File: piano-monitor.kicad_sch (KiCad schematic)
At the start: 9 parts, among them J2 C14, J3 R, J4 DC, J5 230AC, J6 L

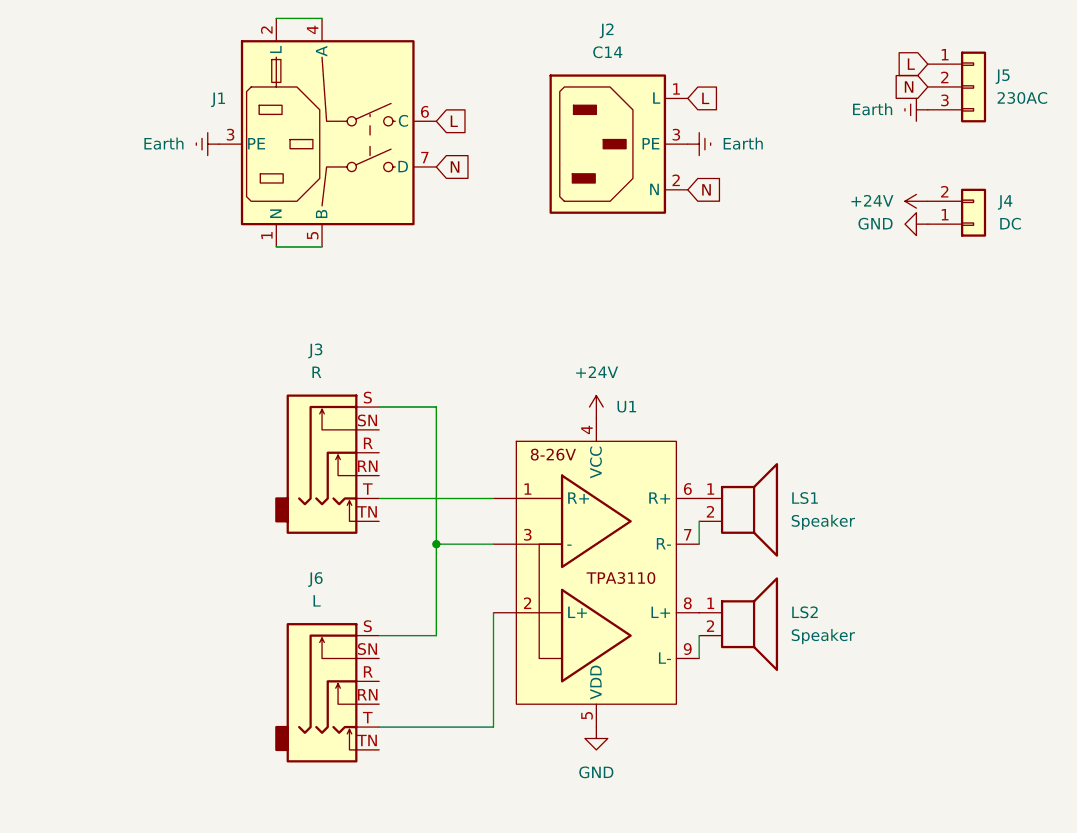
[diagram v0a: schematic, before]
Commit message: Update Schematic
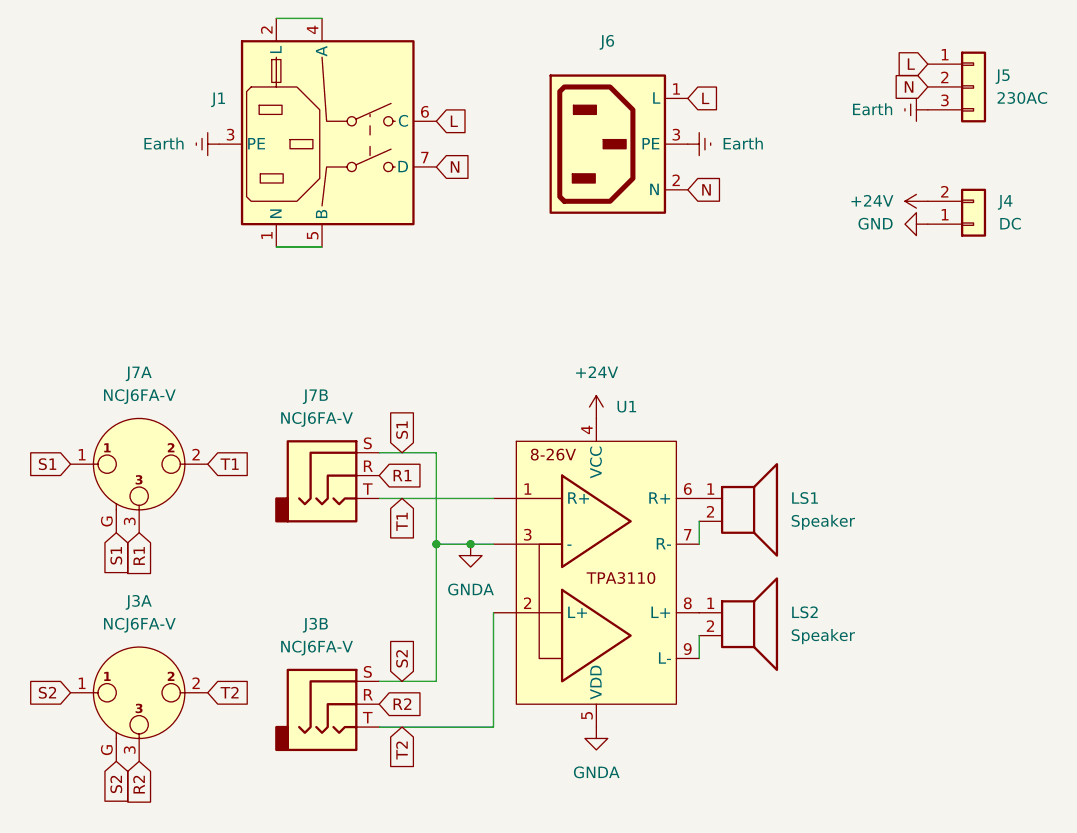
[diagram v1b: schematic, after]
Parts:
- removed J2: C14, symbol Connector:IEC_60320_C14_Receptacle
- removed J3: R, symbol Connector_Audio:AudioJack3_Switch
- removed J6: L, symbol Connector_Audio:AudioJack3_Switch
- added J3, J7: NCJ6FA-V, Connector_Audio:Jack_XLR-6.35mm_Neutrik_NCJ6FA-V_Vertical, symbol Connector_Audio:NCJ6FA-V
- added J6: ~, c14-outlet:c14-outlet, symbol c14-outlet:c14-outlet
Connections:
- net Earth: now also J6.3 (PE)
- net GND: no longer U1.5 (VDD)
- net L: now also J6.1 (L)
- net N: now also J6.2 (N)
- net GNDA: now reaches U1.3 (-)
- net GNDA: now also U1.5 (VDD), J3.1, J3.G, J3.S, J7.1, J7.G, J7.S
- net T1: now reaches U1.1 (R+)
- net T1: now also J7.2, J7.T
- net T2: now reaches U1.2 (L+)
- net T2: now also J3.2, J3.T
- new net R1: J7.3, J7.R
- new net R2: J3.3, J3.R
